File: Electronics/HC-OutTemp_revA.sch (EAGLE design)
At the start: 27 parts, among them SW1 SWITCH_SLIDE, U1 ATMEGA328P-AU, U2 NRF24L01, U3 TMP102

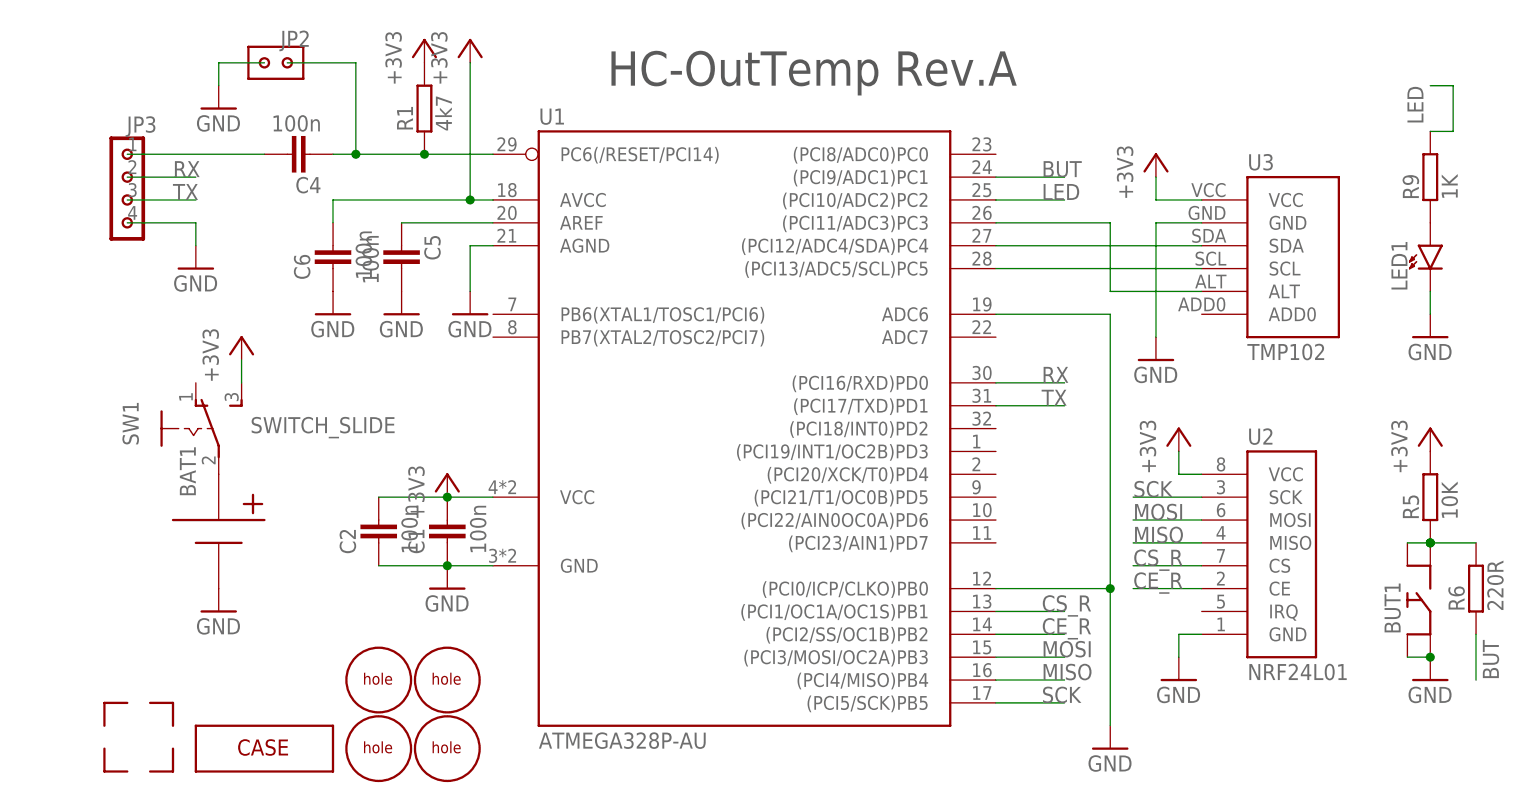
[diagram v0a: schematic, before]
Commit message: modified: PCB
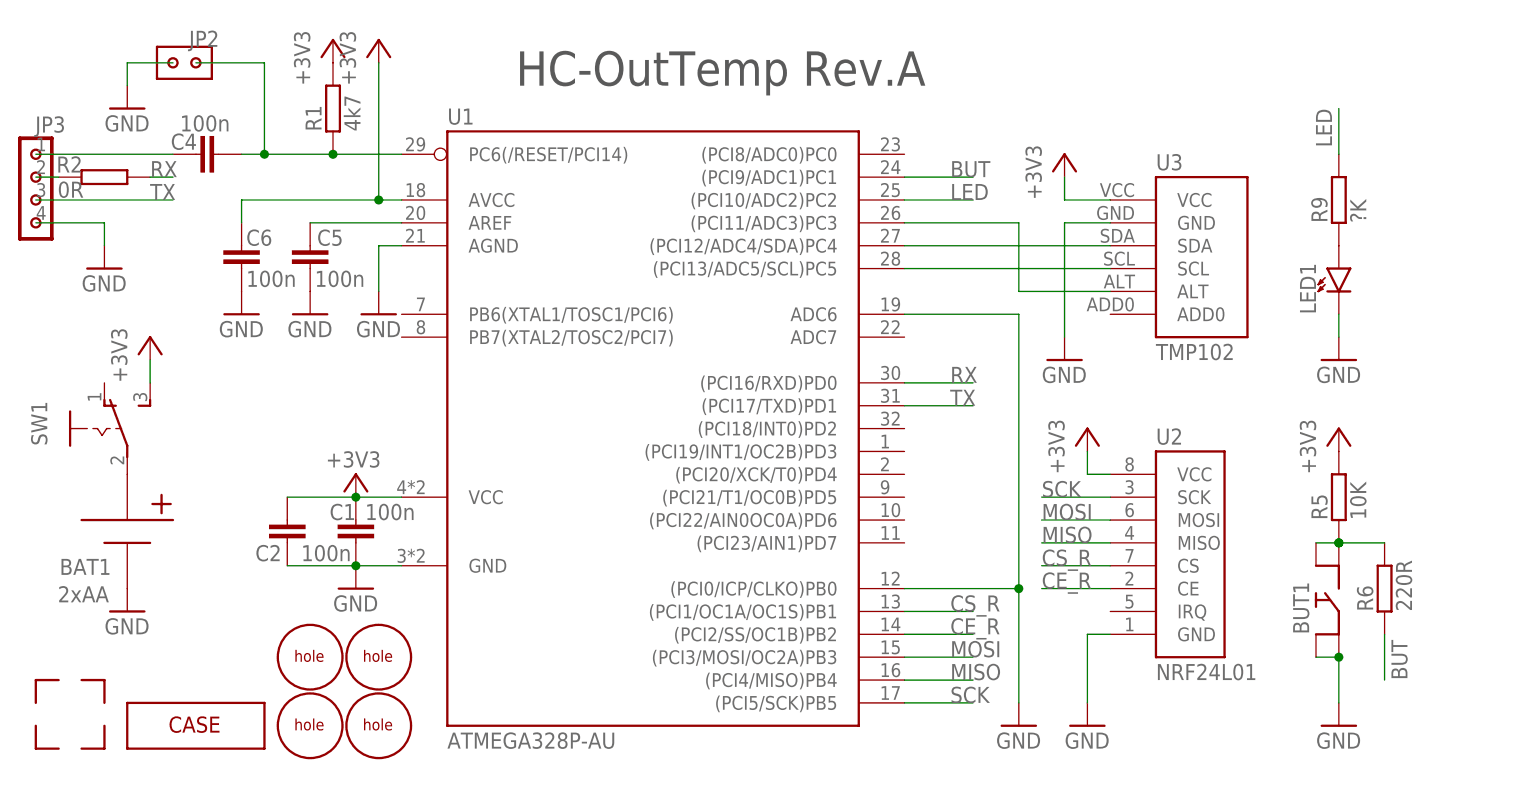
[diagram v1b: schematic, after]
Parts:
- added R2: 0R, 1_domaci:R'2'
- BAT1: value (none) -> 2xAA
- R9: value 1K -> ?K
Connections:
- new net N$8: JP3.2, R2.P$2
- net RX: now also R2.P$1; no longer JP3.2
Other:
- moved on the sheet: BAT1, BUT1, C1, C2, C4, C5, C6, JP2, JP3, LED1, R1, R5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
